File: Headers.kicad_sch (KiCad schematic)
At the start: 4 parts, among them P1 Power Header, P2 Analog Header, P3 Digital Header 02, P4 Digital Header 01

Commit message: add packages
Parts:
- P1, P4: footprint ~ -> Connector_PinSocket_2.54mm:PinSocket_1x08_P2.54mm_Vertical
- P2: footprint ~ -> Connector_PinSocket_2.54mm:PinSocket_1x06_P2.54mm_Vertical
- P3: footprint ~ -> Connector_PinSocket_2.54mm:PinSocket_1x10_P2.54mm_Vertical
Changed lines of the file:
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@@
       (effects (font (size 1.524 1.524)) (justify left))
     )
-    (property "Footprint" "~" (at 158.75 59.69 0)
-      (effects (font (size 1.524 1.524)))
+    (property "Footprint" "Connector_PinSocket_2.54mm:PinSocket_1x08_P2.54mm_Vertical" (at 158.75 59.69 0)
+      (effects (font (size 1.524 1.524)) hide)
     )
     (property "Datasheet" "http://sullinscorp.com/catalogs/101_PAGE114-115_.100_FEMALE_HDR.pdf" (at 158.75 59.69 0)
@@
       (effects (font (size 1.524 1.524)) (justify left))
     )
-    (property "Footprint" "~" (at 158.75 113.03 0)
-      (effects (font (size 1.524 1.524)))
+    (property "Footprint" "Connector_PinSocket_2.54mm:PinSocket_1x10_P2.54mm_Vertical" (at 158.75 113.03 0)
+      (effects (font (size 1.524 1.524)) hide)
     )
     (property "Datasheet" "http://sullinscorp.com/catalogs/101_PAGE114-115_.100_FEMALE_HDR.pdf" (at 158.75 113.03 0)
@@
       (effects (font (size 1.524 1.524)) (justify left))
     )
-    (property "Footprint" "~" (at 158.75 86.36 0)
-      (effects (font (size 1.524 1.524)))
+    (property "Footprint" "Connector_PinSocket_2.54mm:PinSocket_1x06_P2.54mm_Vertical" (at 158.75 86.36 0)
+      (effects (font (size 1.524 1.524)) hide)
     )
     (property "Datasheet" "http://sullinscorp.com/catalogs/101_PAGE114-115_.100_FEMALE_HDR.pdf" (at 158.75 86.36 0)
@@
       (effects (font (size 1.524 1.524)) (justify left))
     )
-    (property "Footprint" "~" (at 158.75 139.7 0)
-      (effects (font (size 1.524 1.524)))
+    (property "Footprint" "Connector_PinSocket_2.54mm:PinSocket_1x08_P2.54mm_Vertical" (at 158.75 139.7 0)
+      (effects (font (size 1.524 1.524)) hide)
     )
     (property "Datasheet" "http://sullinscorp.com/catalogs/101_PAGE114-115_.100_FEMALE_HDR.pdf" (at 158.75 139.7 0)

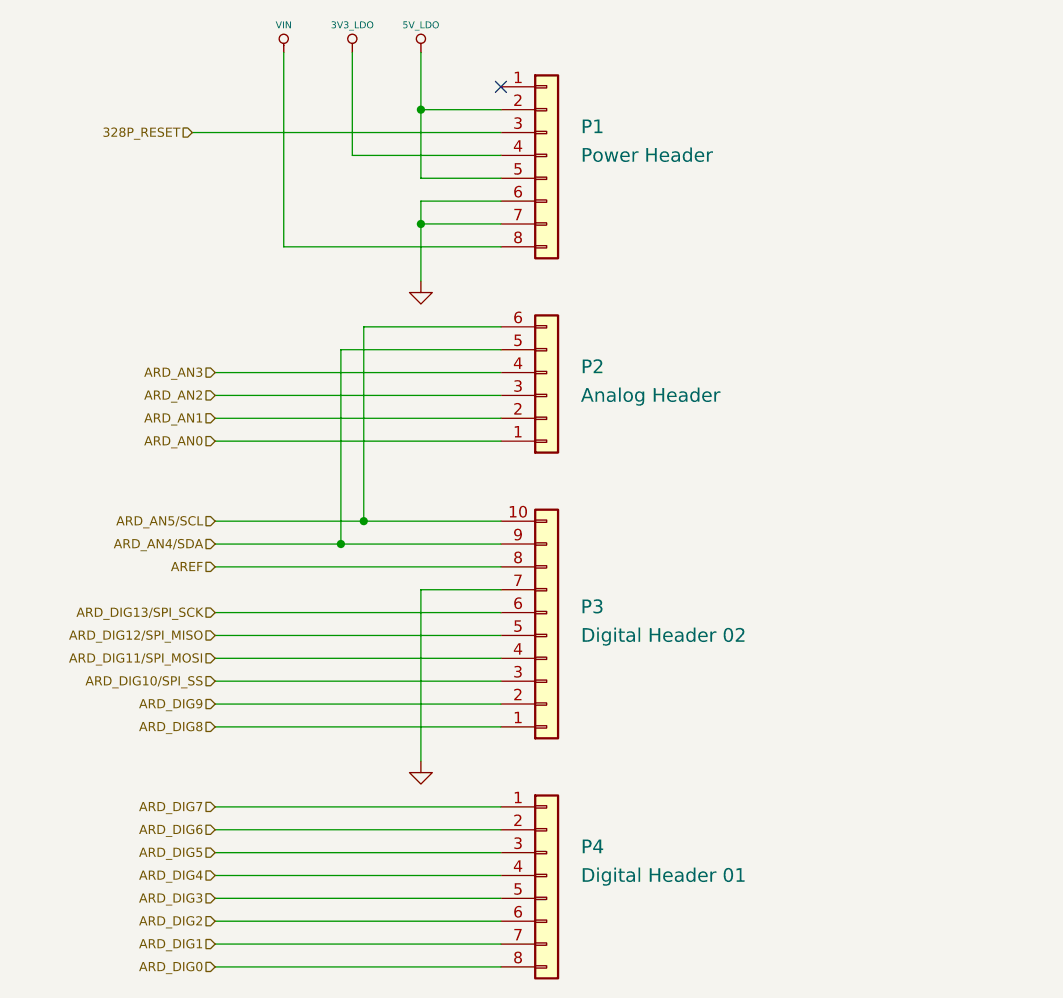
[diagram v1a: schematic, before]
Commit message: change power symbols and Arduino header
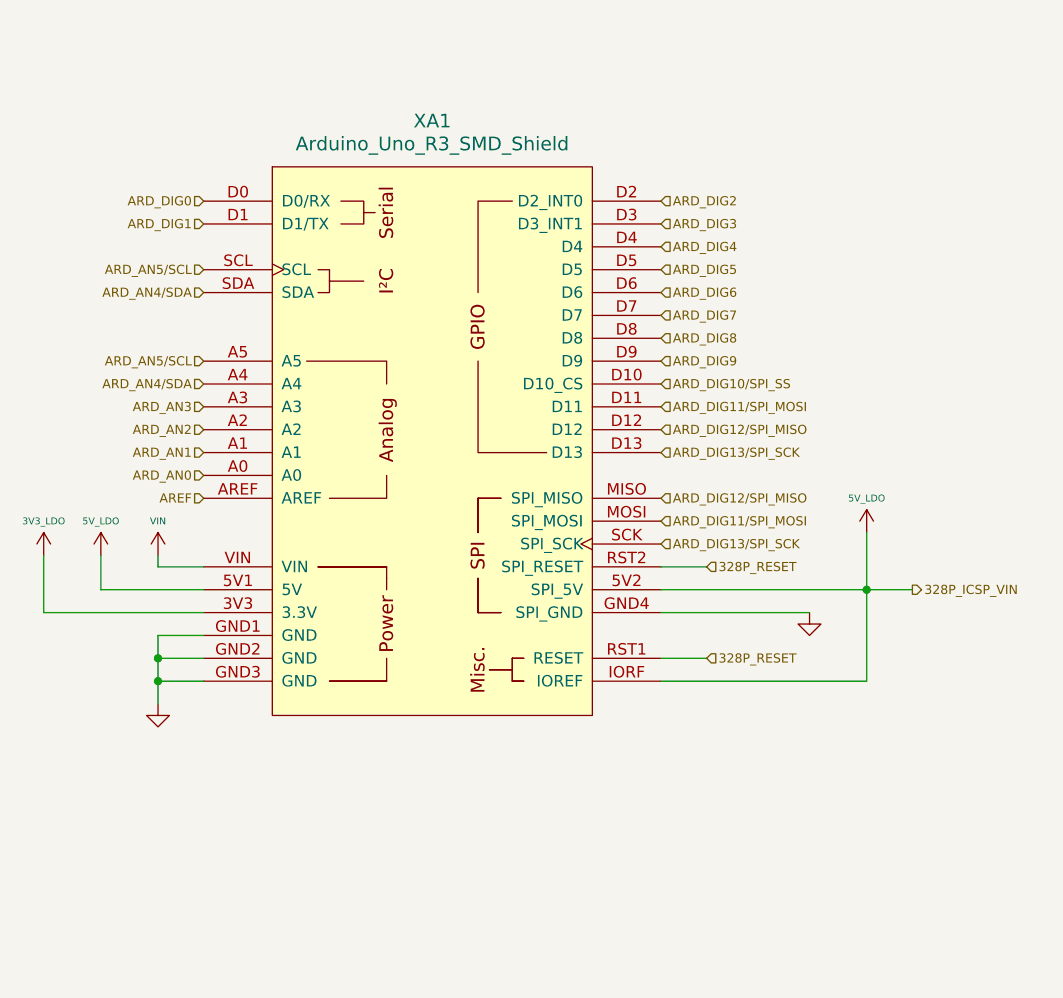
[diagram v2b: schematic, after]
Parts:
- removed P1: Power Header, Connector_PinSocket_2.54mm:PinSocket_1x08_P2.54mm_Vertical, symbol Connector_Generic:Conn_01x08
- removed P2: Analog Header, Connector_PinSocket_2.54mm:PinSocket_1x06_P2.54mm_Vertical, symbol Connector_Generic:Conn_01x06
- removed P3: Digital Header 02, Connector_PinSocket_2.54mm:PinSocket_1x10_P2.54mm_Vertical, symbol Connector_Generic:Conn_01x10
- removed P4: Digital Header 01, Connector_PinSocket_2.54mm:PinSocket_1x08_P2.54mm_Vertical, symbol Connector_Generic:Conn_01x08
- added XA1: Arduino_Uno_R3_SMD_Shield, User Custom Footprint:Arduino_Uno_R3_MountingHole, symbol PCM_arduino-library:Arduino_Uno_R3_SMD_Shield
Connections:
- net 328P_RESET: now also XA1.RST1 (RESET), XA1.RST2 (SPI_RESET)
- net ARD_AN0: now also XA1.A0
- net ARD_AN1: now also XA1.A1
- net ARD_AN2: now also XA1.A2
- net ARD_AN3: now also XA1.A3
- net ARD_AN4/SDA: now also XA1.A4, XA1.SDA
- net ARD_AN5/SCL: now also XA1.A5, XA1.SCL
- net ARD_DIG0: now also XA1.D0 (D0/RX)
- net ARD_DIG1: now also XA1.D1 (D1/TX)
- net ARD_DIG10/SPI_SS: now also XA1.D10 (D10_CS)
- net ARD_DIG11/SPI_MOSI: now also XA1.D11, XA1.MOSI (SPI_MOSI)
- net ARD_DIG12/SPI_MISO: now also XA1.D12, XA1.MISO (SPI_MISO)
- net ARD_DIG13/SPI_SCK: now also XA1.D13, XA1.SCK (SPI_SCK)
- net ARD_DIG2: now also XA1.D2 (D2_INT0)
- net ARD_DIG3: now also XA1.D3 (D3_INT1)
- net ARD_DIG4: now also XA1.D4
- net ARD_DIG5: now also XA1.D5
- net ARD_DIG6: now also XA1.D6
- net ARD_DIG7: now also XA1.D7
- net ARD_DIG8: now also XA1.D8
- net ARD_DIG9: now also XA1.D9
- net AREF: now also XA1.AREF
- net GND: now also XA1.GND1 (GND), XA1.GND2 (GND), XA1.GND3 (GND), XA1.GND4 (SPI_GND)
- new net +3.3V: XA1.3V3 (3.3V)
- new net +5V: XA1.5V1 (5V), XA1.5V2 (SPI_5V), XA1.IORF (IOREF)
- new net VBUS: XA1.VIN
- no-connect marks 1 -> 0
